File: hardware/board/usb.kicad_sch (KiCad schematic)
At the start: 22 parts, among them J501 USB_B_Micro, J502 USB_C_Receptacle_PowerOnly_6P, P501 USB_C_Plug_USB2.0, U501 AP22653W6, U502 FSUSB42MX, U503 TPS259531DSGR

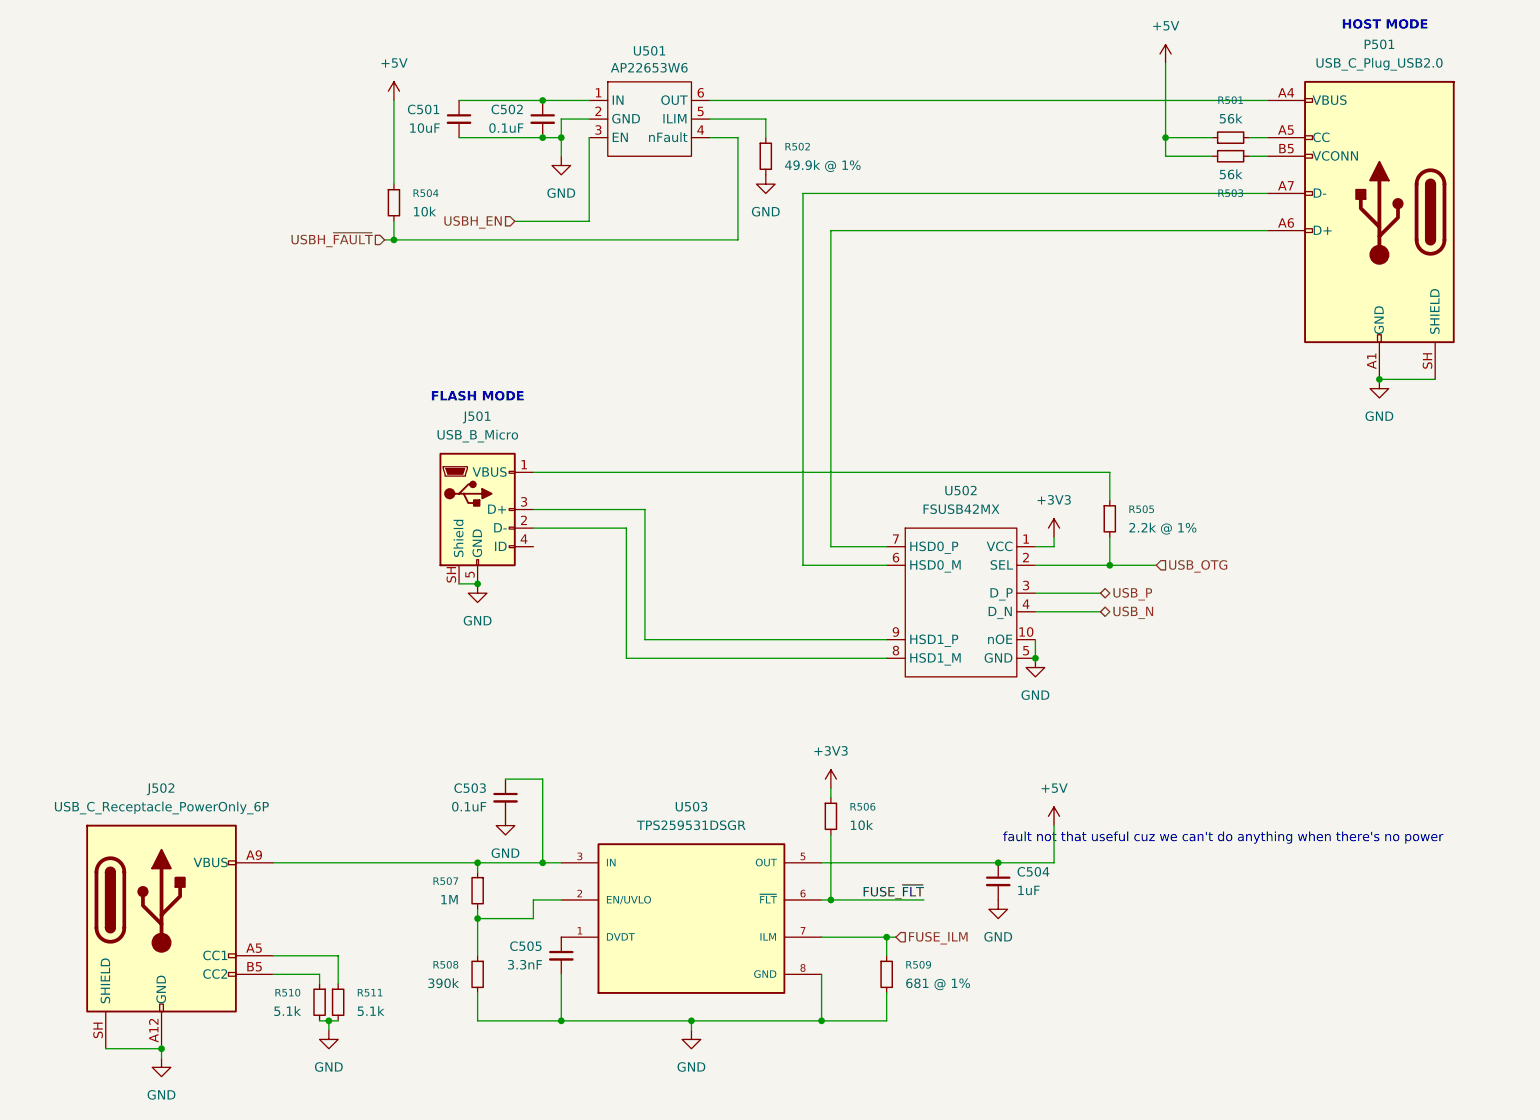
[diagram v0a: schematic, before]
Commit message: some big tim routing
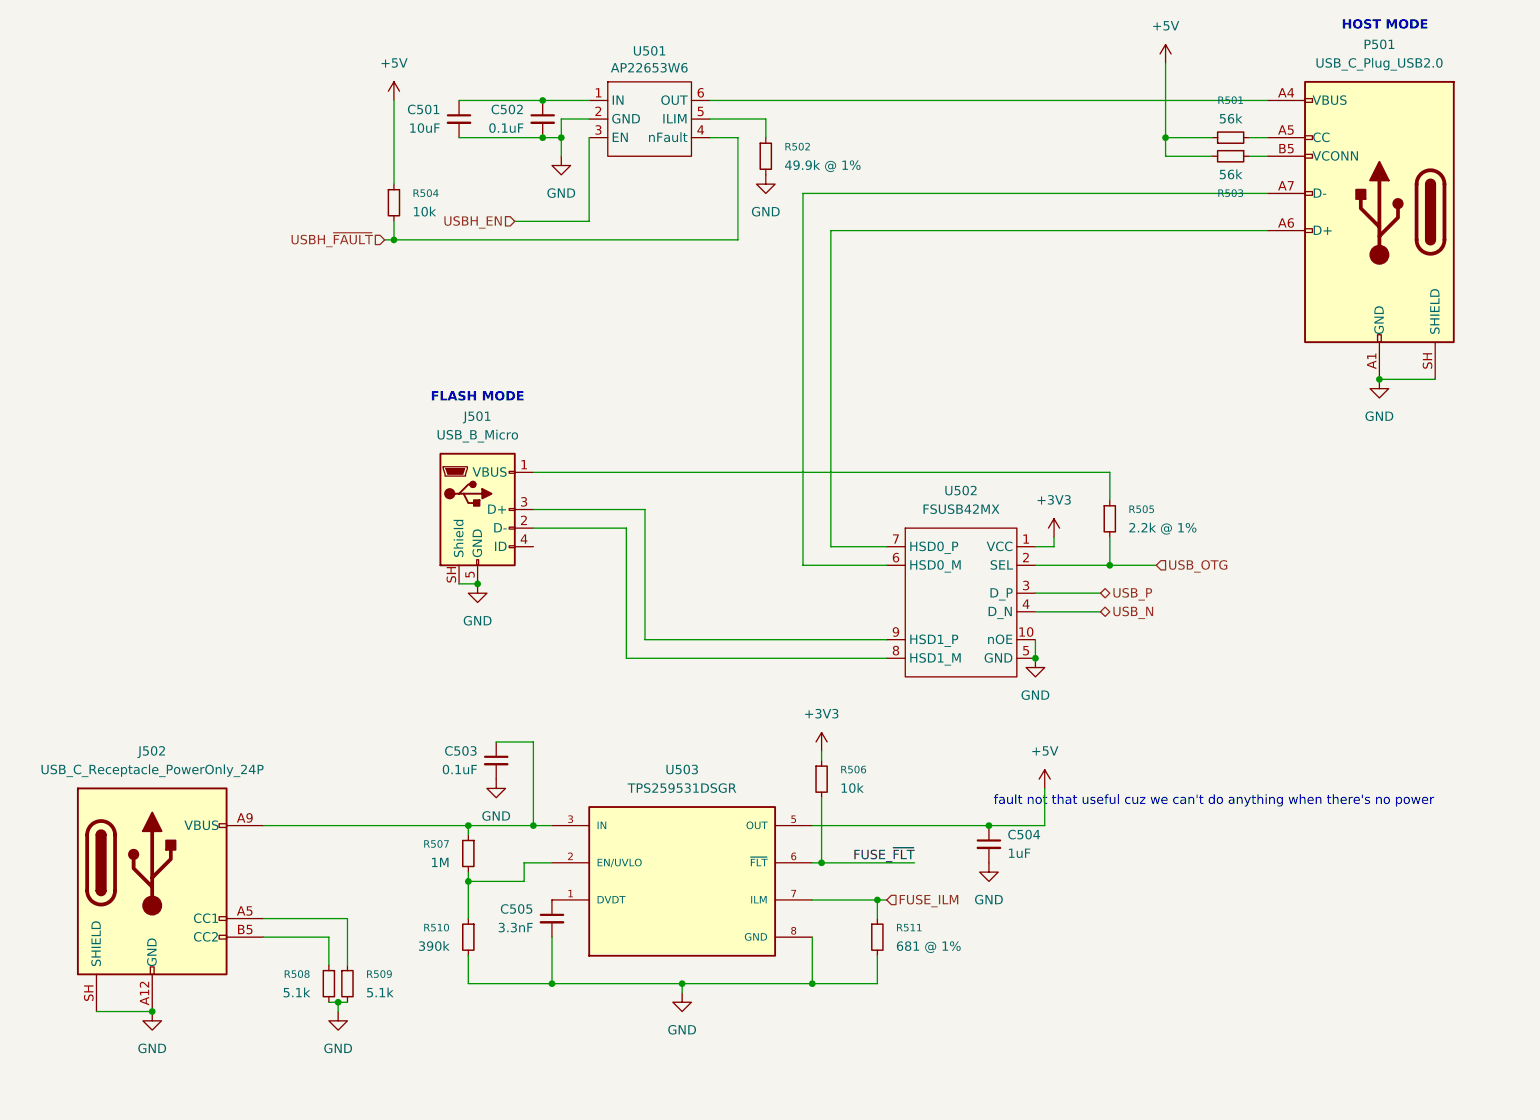
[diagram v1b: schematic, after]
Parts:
- removed J502: USB_C_Receptacle_PowerOnly_6P, Connector_USB:USB_C_Receptacle_HRO_TYPE-C-31-M-12, symbol Connector:USB_C_Receptacle_PowerOnly_6P
- added J502: USB_C_Receptacle_PowerOnly_24P, Connector_USB:USB_C_Receptacle_HRO_TYPE-C-31-M-12, symbol Connector:USB_C_Receptacle_PowerOnly_24P
- renumbered R510 to R508, R511 to R509, R508 to R510, R509 to R511
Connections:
- net GND: now also J502.A1 (GND), J502.A12 (GND), J502.B1 (GND), J502.B12 (GND), J502.SH (SHIELD)
- net at C503.1, R507.1, U503.3 (IN)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: now also J502.A4 (VBUS), J502.A9 (VBUS), J502.B4 (VBUS), J502.B9 (VBUS)
- net at R509.1: now also J502.A5 (CC1)
- net at R508.1: now also J502.B5 (CC2)
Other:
- moved on the sheet: C503, C504, C505, R506, R507, R508, R509, R510, R511, U503
